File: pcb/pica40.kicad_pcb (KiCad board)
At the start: 2 copper layers, 135 x 93.7 mm, 67 parts, among them SW1 SW_PUSH, SW10 SW_PUSH, SW11 SW_PUSH, SW12 SW_PUSH, SW13 SW_PUSH, SW14 SW_PUSH, SW15 SW_PUSH, SW16 SW_PUSH, SW17 SW_PUSH, SW18 SW_PUSH, SW19 SW_PUSH, SW2 SW_PUSH, SW20 SW_PUSH, SW3 SW_PUSH, SW4 SW_PUSH, SW5 SW_PUSH, SW6 SW_PUSH, SW7 SW_PUSH, SW8 SW_PUSH, SW9 SW_PUSH, U1 ProMicro

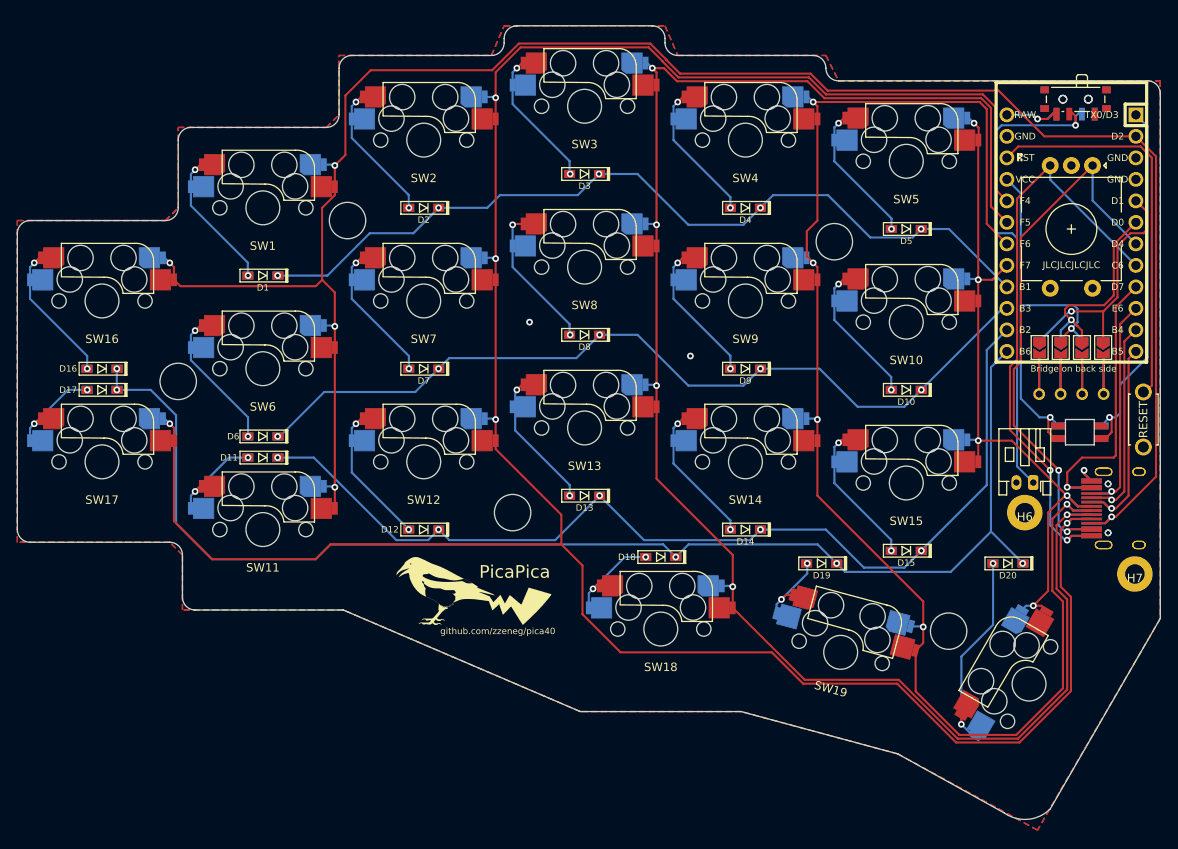
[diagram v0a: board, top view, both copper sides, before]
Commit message: update and reroute
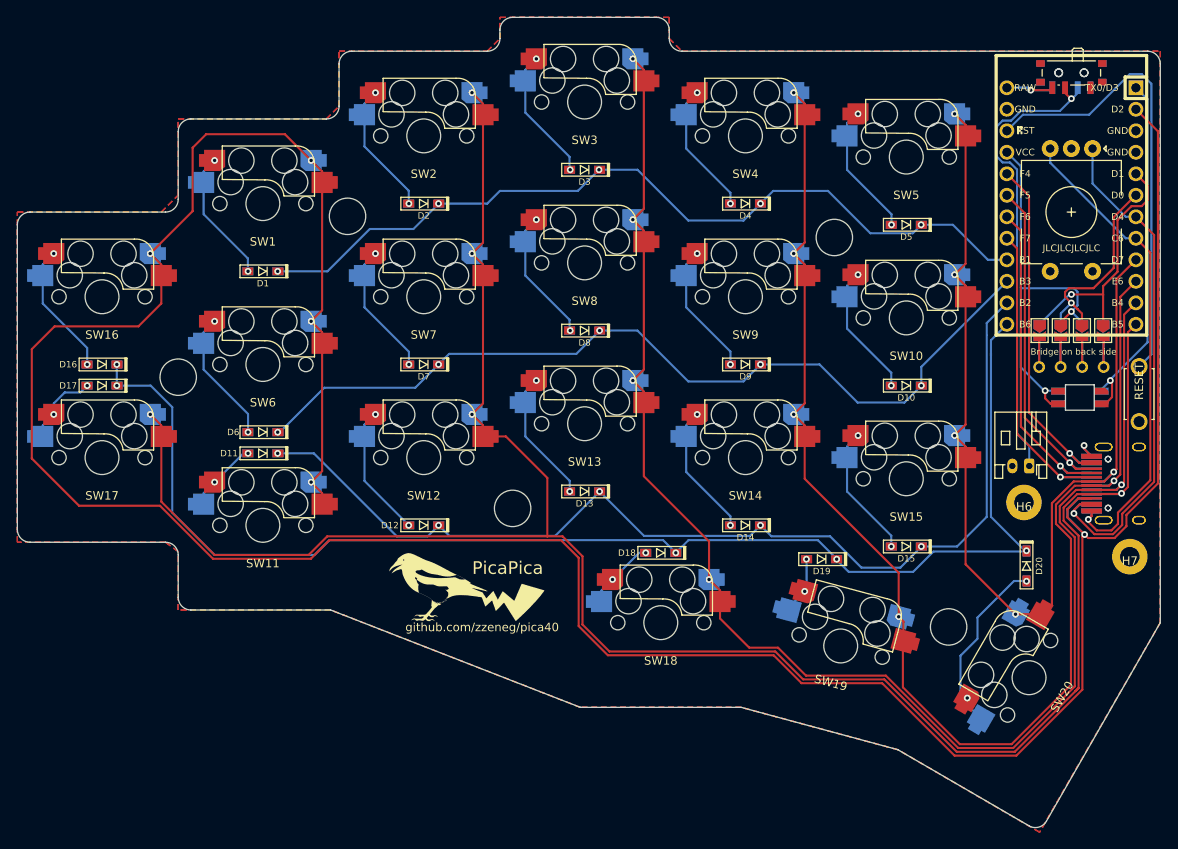
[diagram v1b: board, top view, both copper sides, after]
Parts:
- moved LED1 4.10 mm to (194.0, 95.4)
- moved OLED1 3.20 mm to (193.0, 91.8)
- moved U1 3.20 mm to (193.0, 72.8)
- moved BATTSW1 3.16 mm to (193.0, 57.4)
- moved BATTSW2 3.16 mm to (193.0, 57.4)
- moved RESET1 3.04 mm to (201.0, 95.0)
- moved USB1 2.93 mm to (203.6, 105.6)
- moved USB2 2.93 mm to (203.6, 105.6)
- moved D20 2.22 mm to (187.7, 115.3), turned to -90 degrees
- moved H7 2.14 mm to (199.9, 114.2)
- moved BATTCONN1 2.02 mm to (188.0, 103.5)
- moved JP1 2.00 mm to (189.2, 87.5)
- moved JP2 2.00 mm to (189.2, 87.5)
- moved JP3 2.00 mm to (191.8, 87.5)
- moved JP4 2.00 mm to (191.8, 87.5)
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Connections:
- U1 pad 10: row6 -> col3
- U1 pad 11: row5 -> col2
- U1 pad 12: row4 -> col1
- U1 pad 17: col4 -> row4
- U1 pad 18: col3 -> row5
- U1 pad 19: col2 -> row6
- U1 pad 20: col1 -> row7
- U1 pad 9: row7 -> col4
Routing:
- net col0: track 229.9 -> 349.5 mm
- net col1: track 301.5 -> 255.3 mm
- net col4: track 85.8 -> 119.2 mm
- net col2: track 204.9 -> 180.1 mm
- net row4: track 24.3 -> 38.2 mm
- net row5: track 26.7 -> 40.1 mm
- net ENCB: track 71.3 -> 58.4 mm, vias 2 -> 1
- net row6: track 28.3 -> 40.4 mm
- net col3: track 169.7 -> 160.8 mm
- net RESET: track 46.6 -> 54.3 mm
- net row7: track 35.0 -> 42.2 mm
- net row3: track 154.2 -> 159.9 mm
- net row2: track 118.9 -> 124.5 mm
- net ENCA: track 67.3 -> 62.5 mm, vias 2 -> 1
- net BATT: track 58.4 -> 54.7 mm
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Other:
- board size 135 x 93.7 mm -> 135 x 95.7 mm
